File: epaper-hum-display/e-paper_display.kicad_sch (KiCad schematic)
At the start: 22 parts, among them Q1 Si1308EDL, Q2 PMV65XP,215

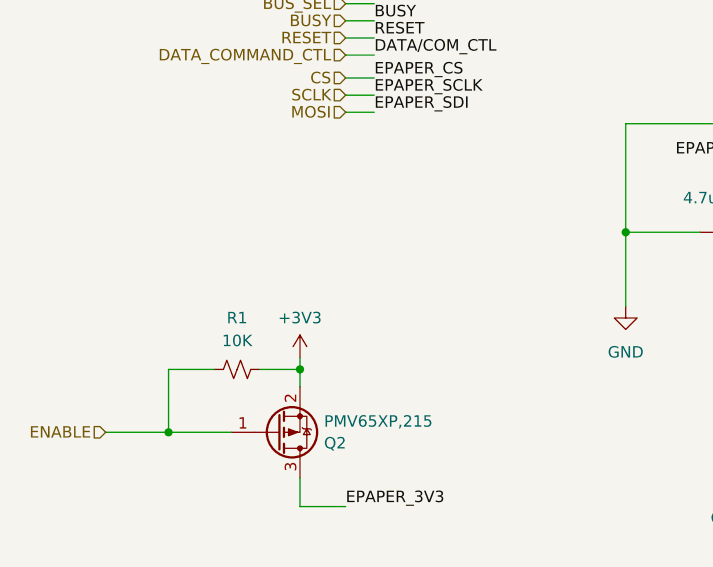
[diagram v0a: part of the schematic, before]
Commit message: WIP
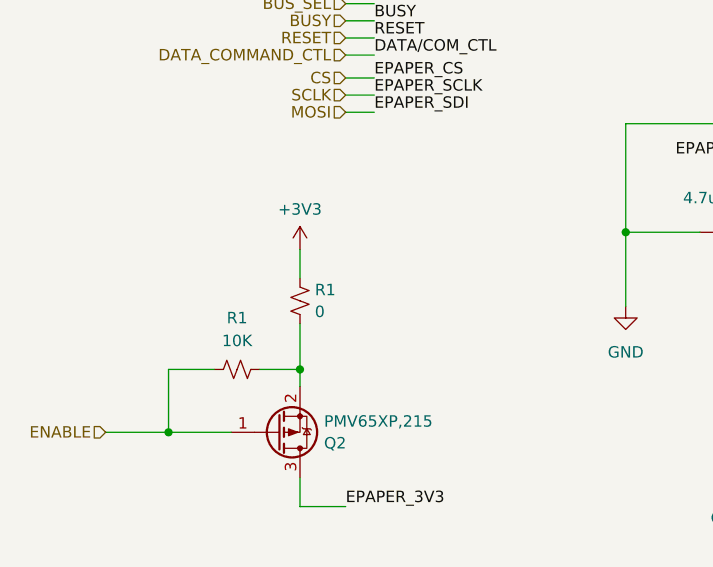
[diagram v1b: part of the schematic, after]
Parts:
- added R1: 0, symbol Device:R_Small_US
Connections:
- net +3V3: now also R1.2; no longer Q2.2 (S), R1.2
- new net: Q2.2 (S), R1.1, R1.2
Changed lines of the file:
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@@
     (stroke (width 0) (type default))
   )
-  (wire (pts (xy 76.2 100.33) (xy 76.2 101.6))
+  (wire (pts (xy 76.2 96.52) (xy 76.2 101.6))
     (stroke (width 0) (type default))
   )
@@
   )
   (wire (pts (xy 180.975 120.015) (xy 180.975 124.46))
+    (stroke (width 0) (type default))
+  )
+  (wire (pts (xy 76.2 88.265) (xy 76.2 91.44))
     (stroke (width 0) (type default))
   )
@@
     )
   )
-  (symbol (lib_id "power:+3V3") (at 76.2 100.33 0) (unit 1)
+  (symbol (lib_id "power:+3V3") (at 76.2 88.265 0) (unit 1)
     (in_bom yes) (on_board yes) (dnp no)
-    (property "Reference" "#PWR05" (at 76.2 104.14 0)
-      (effects (font (size 1.27 1.27)) hide)
-    )
-    (property "Value" "+3V3" (at 76.2 95.885 0)
-      (effects (font (size 1.27 1.27)))
-    )
-    (property "Footprint" "" (at 76.2 100.33 0)
-      (effects (font (size 1.27 1.27)) hide)
-    )
-    (property "Datasheet" "" (at 76.2 100.33 0)
+    (property "Reference" "#PWR05" (at 76.2 92.075 0)
+      (effects (font (size 1.27 1.27)) hide)
+    )
+    (property "Value" "+3V3" (at 76.2 83.82 0)
+      (effects (font (size 1.27 1.27)))
+    )
+    (property "Footprint" "" (at 76.2 88.265 0)
+      (effects (font (size 1.27 1.27)) hide)
+    )
+    (property "Datasheet" "" (at 76.2 88.265 0)
       (effects (font (size 1.27 1.27)) hide)
     )
@@
         )
       )
+    )
+  )
+  (symbol (lib_id "Device:R_Small_US") (at 76.2 93.98 180) (unit 1)
+    (in_bom yes) (on_board yes) (dnp no) (fields_autoplaced)
+    (property "Reference" "R1" (at 77.851 92.7679 0)
+      (effects (font (size 1.27 1.27)) (justify right))
+    )
+    (property "Value" "0" (at 77.851 95.1921 0)
+      (effects (font (size 1.27 1.27)) (justify right))
+    )
+    (property "Footprint" "" (at 76.2 93.98 0)
+      (effects (font (size 1.27 1.27)) hide)
+    )
+    (property "Datasheet" "~" (at 76.2 93.98 0)
+      (effects (font (size 1.27 1.27)) hide)
+    )
+    (pin "1")
+    (pin "2")
+    (instances
+      (project "epaper-hum-display"
+        (path "/e8301e0c-f140-47c2-97ee-69a5a204efef"
+          (reference "R1") (unit 1)
+        )
+        (path "/e8301e0c-f140-47c2-97ee-69a5a204efef/3f5106e4-1b1e-45fa-91c4-dc93b9e9dbb4"
+          (reference "R28") (unit 1)
+        )
+      )
